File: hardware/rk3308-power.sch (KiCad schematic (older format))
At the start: 1 part, among them U1000 RK3308

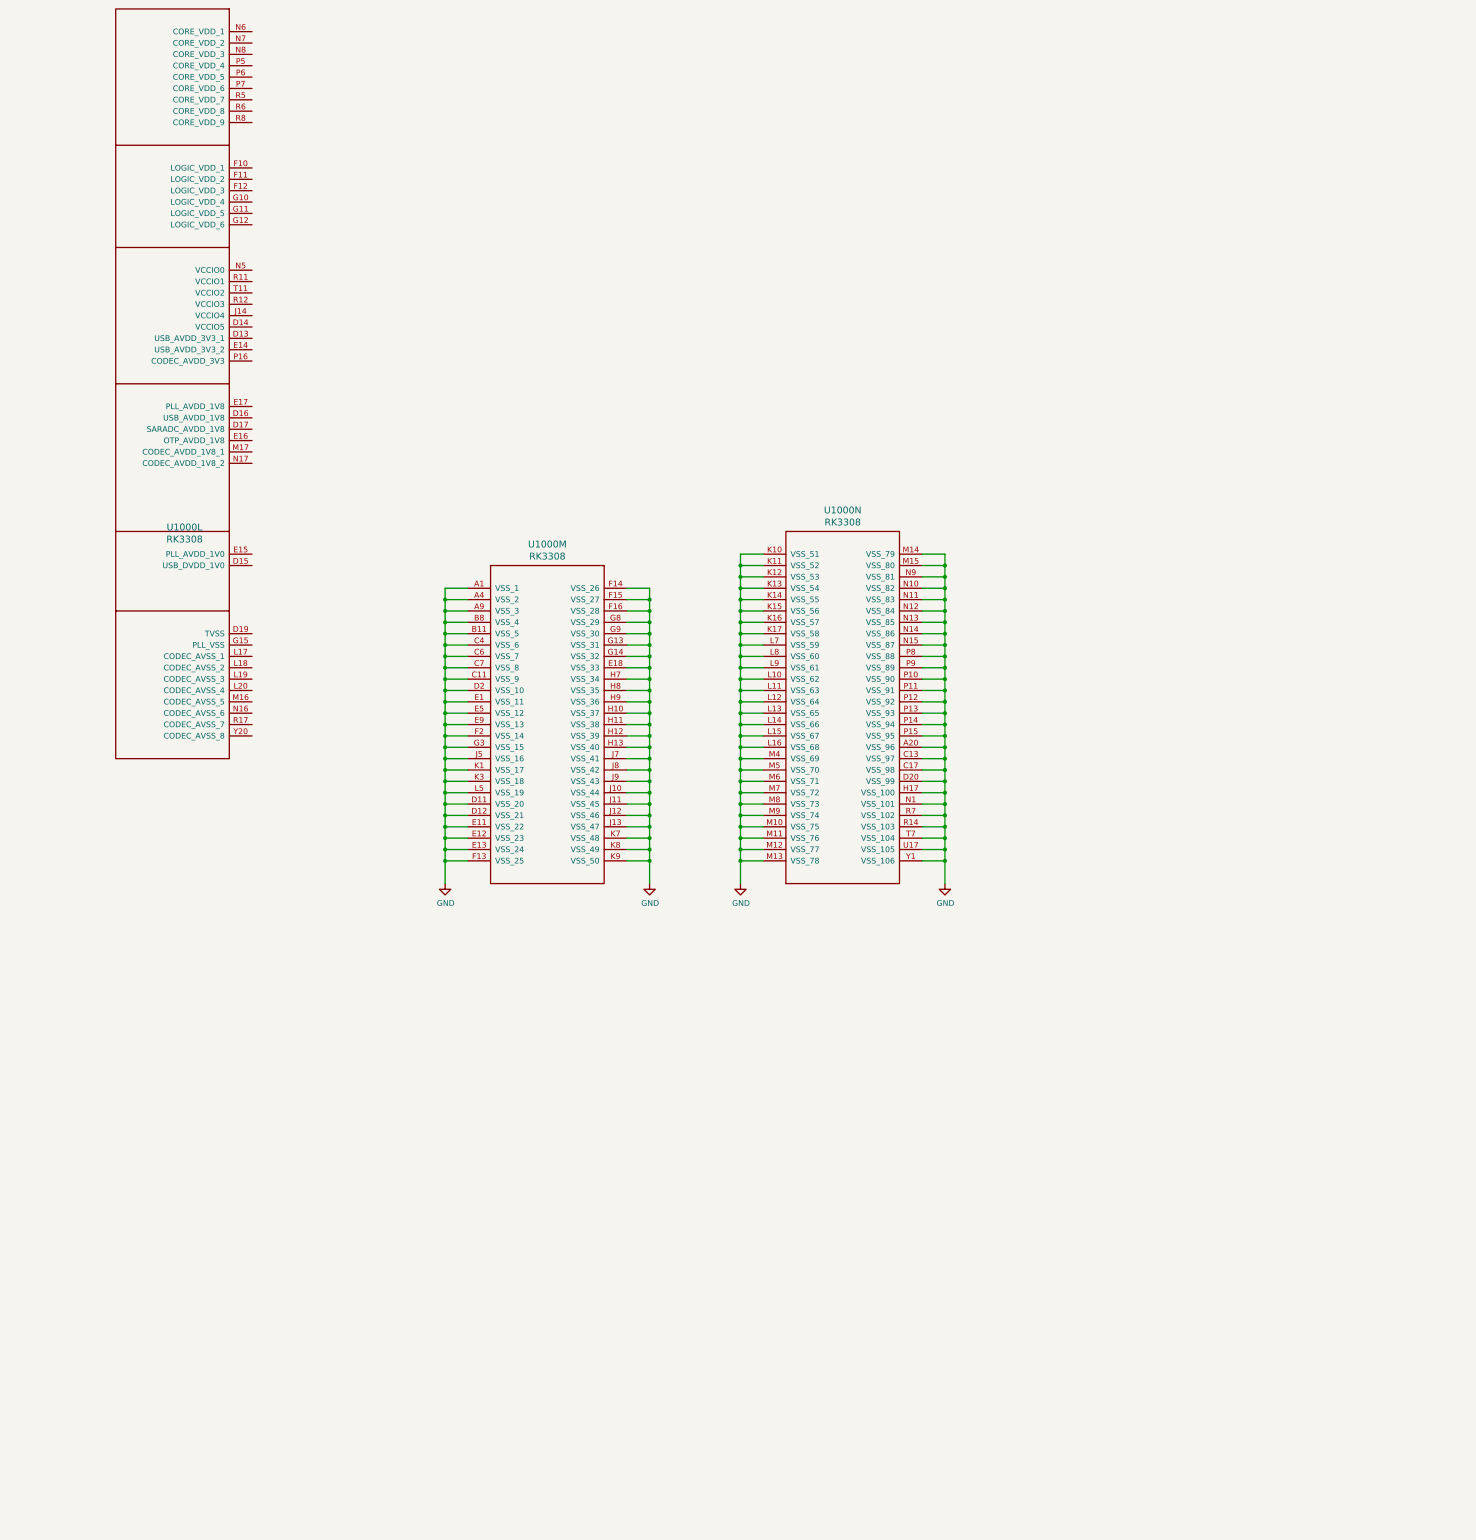
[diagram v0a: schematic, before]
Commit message: wip
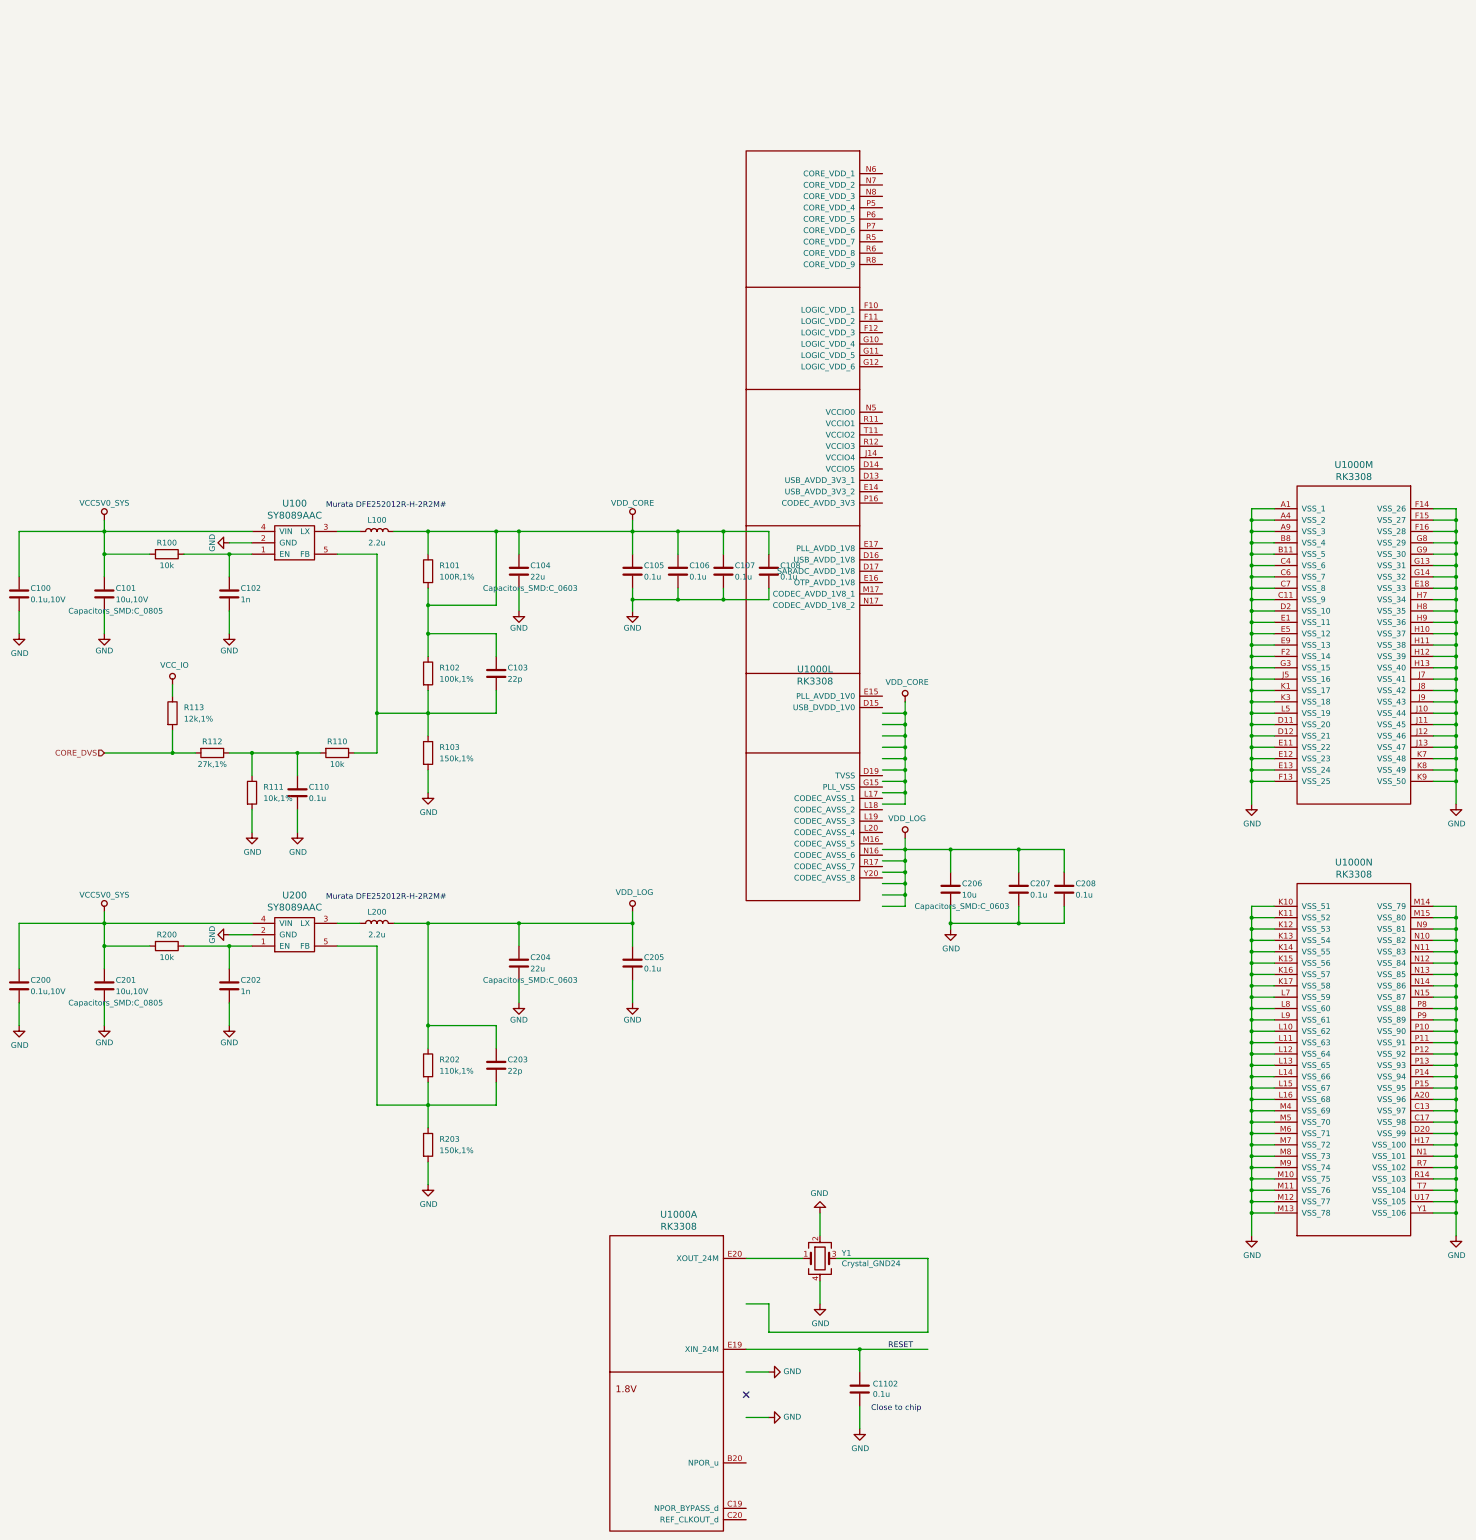
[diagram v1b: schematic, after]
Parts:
- added C100, C200: 0.1u,10V, Capacitors_SMD:C_0402, symbol require-rescue:C
- added C101, C201: 10u,10V, Capacitors_SMD:C_0805, symbol require-rescue:C
- added C102, C202: 1n, Capacitors_SMD:C_0402, symbol require-rescue:C
- added C103, C203: 22p, Capacitors_SMD:C_0402, symbol require-rescue:C
- added C104, C204: 22u, Capacitors_SMD:C_0603, symbol require-rescue:C
- added C105, C106, C107, C108, C110, C205, C207, C208: 0.1u, Capacitors_SMD:C_0402, symbol require-rescue:C
- added C1102: 0.1u, Capacitors_SMD:C_0402, symbol Device:C
- added C206: 10u, Capacitors_SMD:C_0603, symbol require-rescue:C
- added L100, L200: 2.2u, require:L_murata_2520, symbol require-rescue:L
- added R100, R110, R200: 10k, Resistors_SMD:R_0402, symbol require-rescue:R
- added R101: 100R,1%, Resistors_SMD:R_0402, symbol require-rescue:R
- added R102: 100k,1%, Resistors_SMD:R_0402, symbol require-rescue:R
- added R103, R203: 150k,1%, Resistors_SMD:R_0402, symbol require-rescue:R
- added R111: 10k,1%, Resistors_SMD:R_0402, symbol require-rescue:R
- added R112: 27k,1%, Resistors_SMD:R_0402, symbol require-rescue:R
- added R113: 12k,1%, Resistors_SMD:R_0402, symbol require-rescue:R
- added R202: 110k,1%, Resistors_SMD:R_0402, symbol require-rescue:R
- added U100, U200: SY8089AAC, TO_SOT_Packages_SMD:SOT-23-5, symbol require:SY8089AAC
- added unit 1 of U1000
- added Y1: Crystal_GND24, Crystals:Crystal_SMD_3225-4pin_3.2x2.5mm, symbol Device:Crystal_GND24
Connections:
- net labels added: CORE_DVS, RESET, VCC5V0_SYS, VCC_IO, VDD_CORE, VDD_LOG
- wire segments 212 -> 369
- no-connect marks 0 -> 1
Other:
- note added: "Close to chip"
- note added: "Murata DFE252012R-H-2R2M#\n"
- moved on the sheet: U1000L, U1000M, U1000N
